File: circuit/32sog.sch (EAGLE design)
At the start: 10 parts, among them IC2 TINY15LP

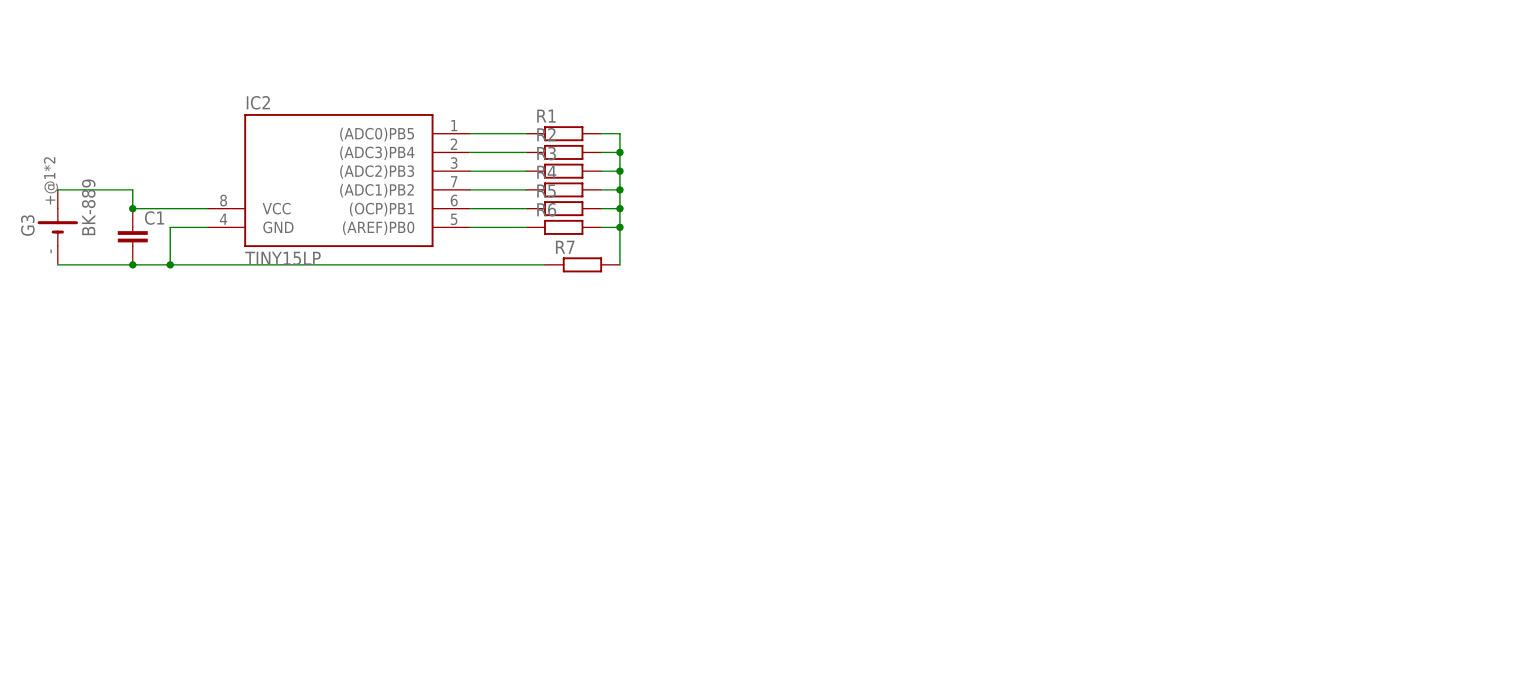
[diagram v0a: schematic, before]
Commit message: Circuit board for a Tic Tac mint box
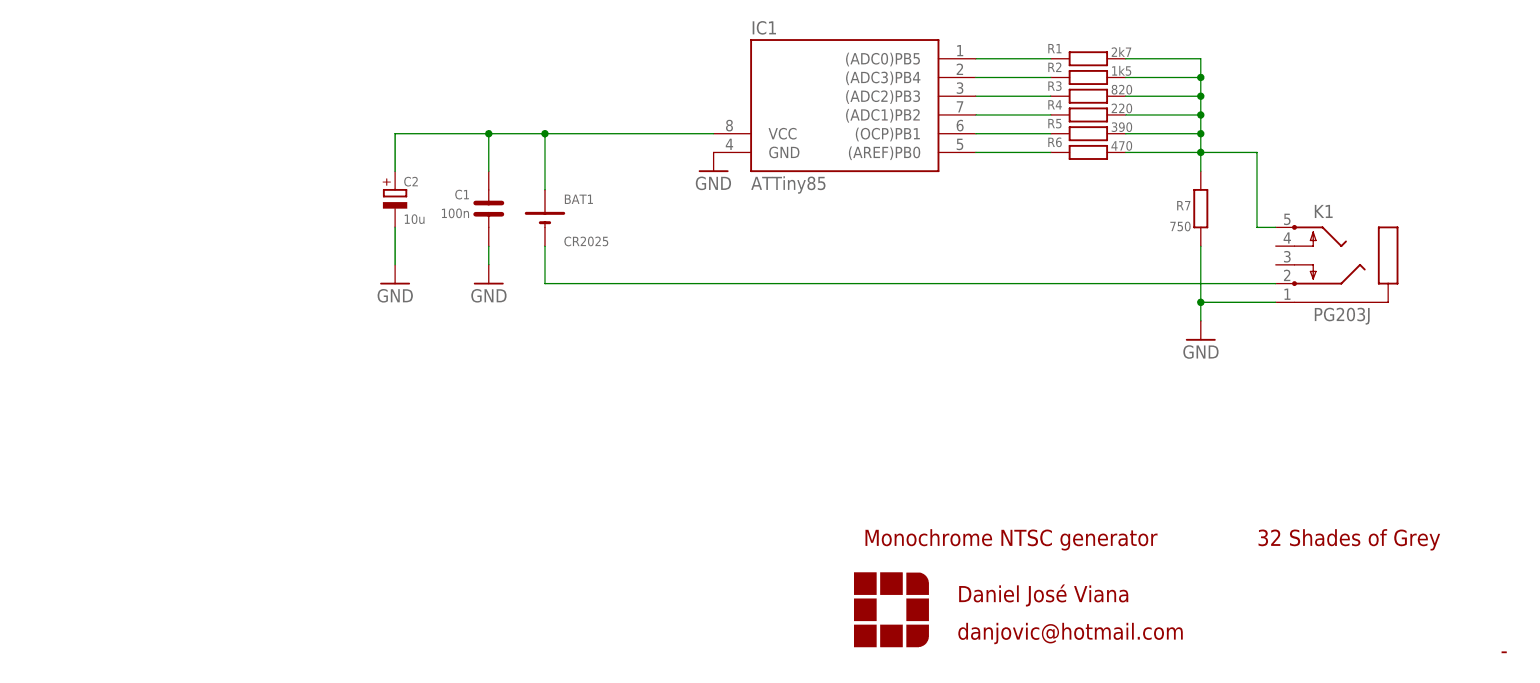
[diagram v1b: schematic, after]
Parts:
- removed G3: BK-889, battery:BK-889
- removed IC2: TINY15LP, atmel:TINY15LP
- added BAT1: CR2025, diversos2:CR2032H1GJ00245
- added C2: 10u, rcl:CPOL-EUE2-4_LARGEPADS
- added IC1: ATTiny85, atmel:TINY15LP
- added K1: PG203J, con-hirschmann:PG203J
- C1: value (none) -> 100n; device rcl:C-EU050-025X075 -> diversos2:CCERAMICO
- R1: value (none) -> 2k7
- R2: value (none) -> 1k5
- R3: value (none) -> 820
- R4: value (none) -> 390
- R5: value (none) -> 220
- R6: value (none) -> 470
- R7: value (none) -> 750
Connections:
- new net GND: C1.P$1, C2.-, IC1.GND, K1.1, R7.2
- net N$1: now also IC1.(ADC0)PB5; no longer IC2.(ADC0)PB5
- net N$2: now also IC1.(ADC2)PB3, R3.1; no longer IC2.(ADC3)PB4, R2.1
- net N$3: now also BAT1.PLUS, C1.P$2, C2.+, IC1.VCC; no longer IC2.(ADC2)PB3, R3.1
- net N$4: now also IC1.(OCP)PB1, R5.1; no longer IC2.(ADC1)PB2, R4.1
- net N$5: now also IC1.(ADC3)PB4, R2.1; no longer IC2.(OCP)PB1, R5.1
- net N$6: now also IC1.(ADC1)PB2, R4.1; no longer IC2.(AREF)PB0, R6.1
- net N$7: now also IC1.(AREF)PB0, R6.1; no longer R1.2, R2.2, R3.2, R4.2, R5.2, R6.2, R7.2
- net N$8: now also K1.5, R1.2, R2.2, R3.2, R4.2, R5.2, R6.2; no longer C1.2, G3.-, IC2.GND
- net N$9: now also BAT1.MINUS, K1.2; no longer C1.1, G3.+, IC2.VCC
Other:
- note added: "-"
- note added: "32 Shades of Grey"
- note added: "Daniel José Viana"
- note added: "Monochrome NTSC generator"
- note added: "danjovic@hotmail.com"
- moved on the sheet: R1, R2, R3, R4, R5, R6, R7
